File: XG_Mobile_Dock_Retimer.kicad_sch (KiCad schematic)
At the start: 263 parts, among them J1 5-1775443-8, J13 39301240, J14 469911008, J2 20455-040E-76, J3 20455-040E-76, J7 CEE016400140111, SW1 SW_Push, U1 DS160PT801ACBR, U2 TPS7A8400ARGRR, U7 TPS7A8400ARGRR

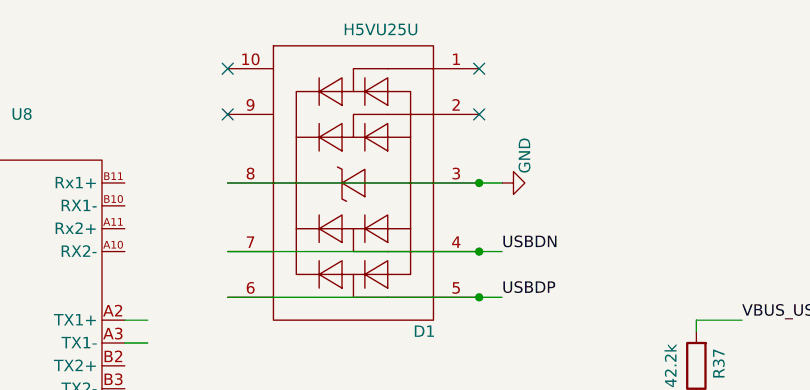
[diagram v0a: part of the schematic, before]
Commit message: eeeee
eeeee
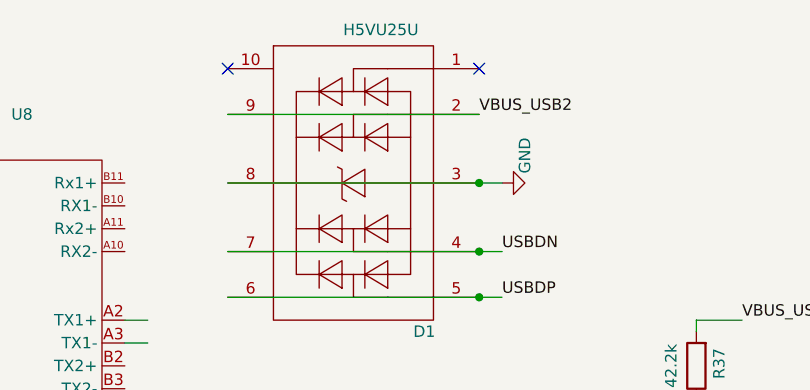
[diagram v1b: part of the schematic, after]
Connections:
- net VBUS_USB2: now also D1.2 (I/O_2), D1.9 (NC)
- no-connect marks 25 -> 23
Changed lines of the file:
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@@
 	)
 	(no_connect
-		(at 215.9 -43.18)
-	)
-	(no_connect
 		(at 544.83 34.29)
 	)
@@
 	)
 	(no_connect
-		(at 243.84 -43.18)
-	)
-	(no_connect
 		(at 514.35 148.59)
 	)
@@
 	(wire
 		(pts
+			(xy 215.9 -43.18) (xy 243.84 -43.18)
+		)
+		(stroke
+			(width 0)
+			(type default)
+		)
+	)
+	(wire
+		(pts
 			(xy 264.16 336.55) (xy 275.59 336.55)
 		)
@@
 		(effects
 			(font
+				(size 1.27 1.27)
+			)
+			(justify left bottom)
+		)
+	)
+	(label "VBUS_USB2"
+		(at 243.84 -43.18 0)
+		(effects
+			(font
